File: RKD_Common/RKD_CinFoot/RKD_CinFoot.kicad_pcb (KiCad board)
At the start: 2 copper layers, 81 x 11.9 mm, 5 parts

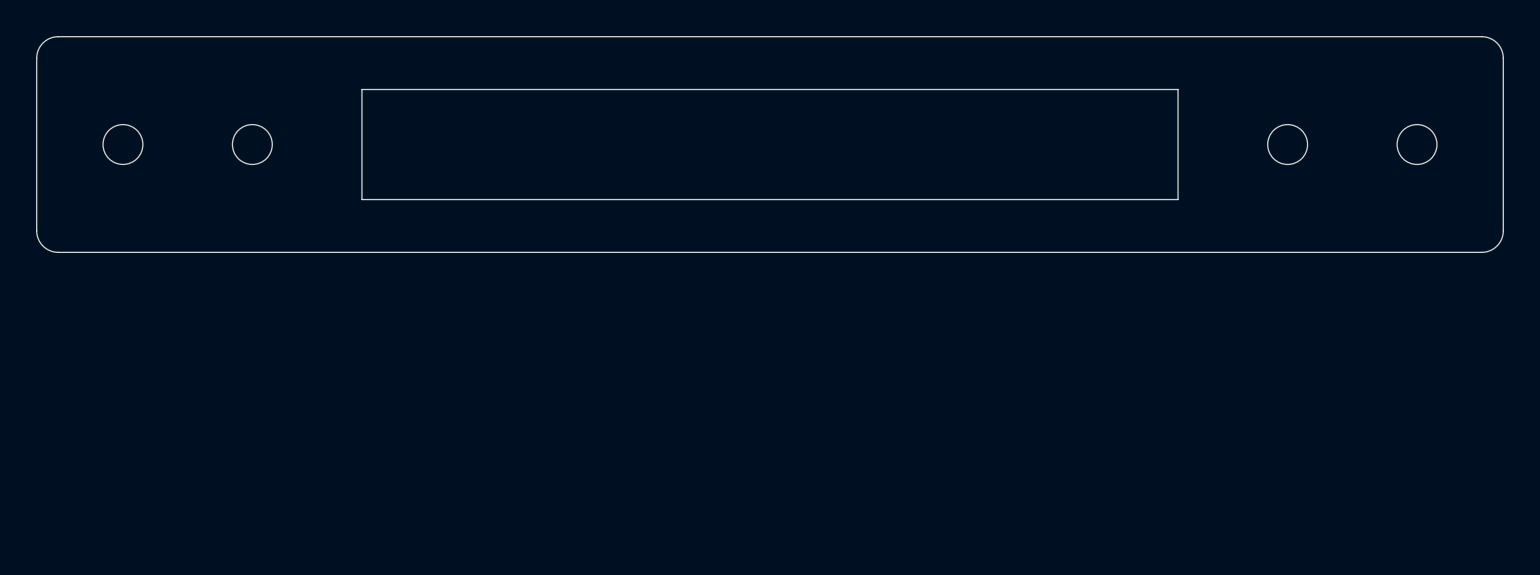
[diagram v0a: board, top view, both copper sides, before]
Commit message: Common UpdateFootPrint
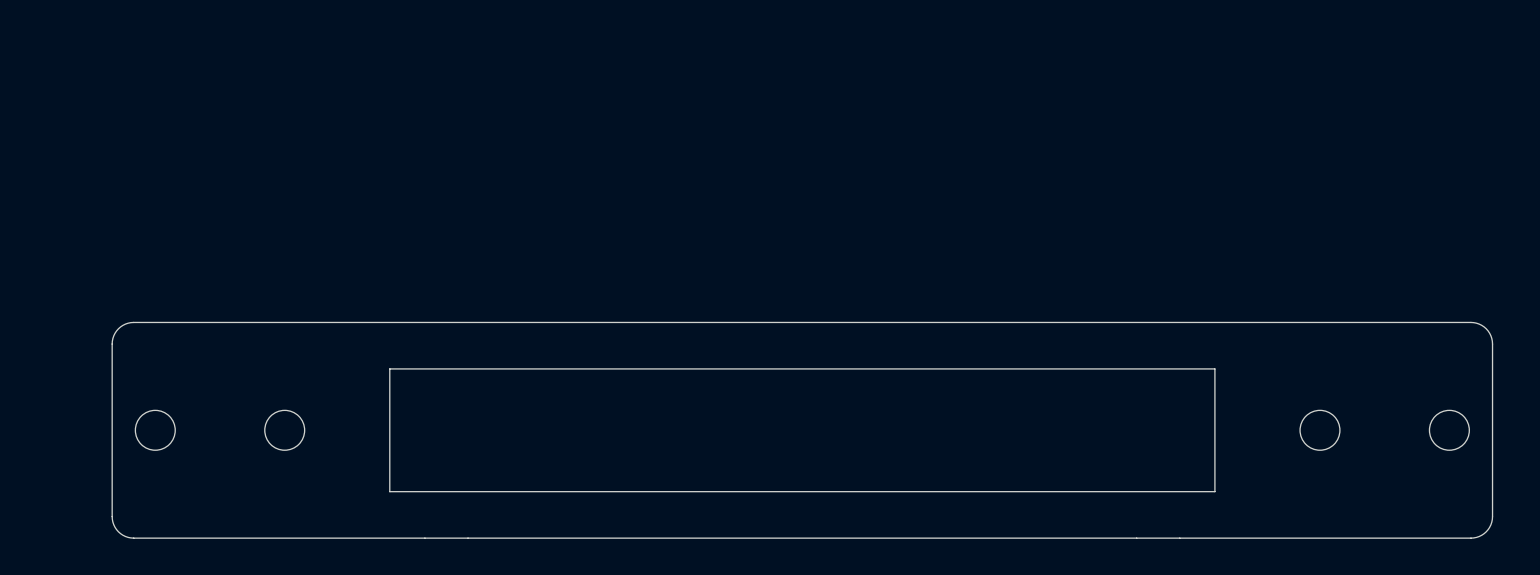
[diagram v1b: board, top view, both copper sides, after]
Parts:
- removed the Ref** at (128.6, 51.2)
- removed the Ref** at (121.4, 51.2)
- removed the Ref** at (64.3, 51.2)
- removed the Ref** at (57.1, 51.2)
- added Ref**: Val**, kbd_Hole:m2_Screw_Hole, F.Cu at (123.2, 67.0)
- added Ref**: Val**, kbd_Hole:m2_Screw_Hole, F.Cu at (58.9, 67.0)
- added Ref**: Val**, kbd_Hole:m2_Screw_Hole, F.Cu at (66.1, 67.0)
- added Ref**: Val**, kbd_Hole:m2_Screw_Hole, F.Cu at (130.4, 67.0)
- moved LED3 15.9 mm to (94.7, 67.0)
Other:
- board size 81 x 11.9 mm -> 76.2 x 11.9 mm
- board text added: "RKD_CinderellaFoot v1.0"
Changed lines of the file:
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@@
 	(footprint "kbd_Hole:m2_Screw_Hole"
 		(layer "F.Cu")
-		(at 128.5875 51.196875)
+		(at 123.229892 66.972702)
 		(descr "Mounting Hole 2.2mm, no annular, M2")
 		(tags "mounting hole 2.2mm no annular m2")
@@
 	(footprint "kbd_Hole:m2_Screw_Hole"
 		(layer "F.Cu")
-		(at 121.44375 51.196875)
+		(at 58.936142 66.972702)
 		(descr "Mounting Hole 2.2mm, no annular, M2")
 		(tags "mounting hole 2.2mm no annular m2")
@@
 	(footprint "kbd_Hole:m2_Screw_Hole"
 		(layer "F.Cu")
-		(at 64.29375 51.196875)
+		(at 66.079892 66.972702)
 		(descr "Mounting Hole 2.2mm, no annular, M2")
 		(tags "mounting hole 2.2mm no annular m2")
@@
 		)
 	)
+	(footprint "Rikkodo_FootPrint:rkd_KeyHall_6wx45_Cinderella"
+		(layer "F.Cu")
+		(at 94.654952 66.972702)
+		(property "Reference" "LED3"
+			(at 6 0.5 0)
+			(layer "F.SilkS")
+			(hide yes)
+			(effects
+				(font
+					(size 1 1)
+					(thickness 0.15)
+				)
+			)
+		)
+		(property "Value" "LED_SK6812MINI-E"
+			(at -5.5 -0.5 0)
+			(layer "F.Fab")
+			(hide yes)
+			(effects
+				(font
+					(size 1 1)
+					(thickness 0.15)
+				)
+			)
+		)
+		(property "Footprint" "Rikkodo_FootPrint:rkd_KeyHall_6wx45_Cinderella"
+			(at 0 0 0)
+			(layer "F.Fab")
+			(hide yes)
+			(effects
+				(font
+					(size 1.27 1.27)
+					(thickness 0.15)
+				)
+			)
+		)
+		(property "Datasheet" ""
+			(at 0 0 0)
+			(layer "F.Fab")
+			(hide yes)
+			(effects
+				(font
+					(size 1.27 1.27)
+					(thickness 0.15)
+				)
+			)
+		)
+		(property "Description" ""
+			(at 0 0 0)
+			(layer "F.Fab")
+			(hide yes)
+			(effects
+				(font
+					(size 1.27 1.27)
+					(thickness 0.15)
+				)
+			)
+		)
+		(attr through_hole)
+		(fp_line
+			(start -22.775 3.3875)
+			(end -22.775 -3.3875)
+			(stroke
+				(width 0.05)
+				(type default)
+			)
+			(layer "Edge.Cuts")
+		)
+		(fp_line
+			(start 22.775 -3.3875)
+			(end -22.775 -3.3875)
+			(stroke
+				(width 0.05)
+				(type default)
+			)
+			(layer "Edge.Cuts")
+		)
+		(fp_line
+			(start 22.775 -3.3875)
+			(end 22.775 3.3875)
+			(stroke
+				(width 0.05)
+				(type default)
+			)
+			(layer "Edge.Cuts")
+		)
+		(fp_line
+			(start 22.775 3.3875)
+			(end -22.775 3.3875)
+			(stroke
+				(width 0.05)
+				(type default)
+			)
+			(layer "Edge.Cuts")
+		)
+	)
 	(footprint "kbd_Hole:m2_Screw_Hole"
 		(layer "F.Cu")
-		(at 57.15 51.196875)
+		(at 130.373642 66.972702)
 		(descr "Mounting Hole 2.2mm, no annular, M2")
 		(tags "mounting hole 2.2mm no annular m2")
@@
 		)
 	)
-	(footprint "Rikkodo_FootPrint:rkd_KeyHall_6wx45_Cinderella"
-		(layer "F.Cu")
-		(at 92.86875 51.196875)
-		(property "Reference" "LED3"
-			(at 6 0.5 0)
-			(layer "F.SilkS")
-			(hide yes)
-			(effects
-				(font
-					(size 1 1)
-					(thickness 0.15)
-				)
-			)
-		)
-		(property "Value" "LED_SK6812MINI-E"
-			(at -5.5 -0.5 0)
-			(layer "F.Fab")
-			(hide yes)
-			(effects
-				(font
-					(size 1 1)
-					(thickness 0.15)
-				)
-			)
-		)
-		(property "Footprint" "Rikkodo_FootPrint:rkd_KeyHall_6wx45_Cinderella"
-			(at 0 0 0)
-			(layer "F.Fab")
-			(hide yes)
-			(effects
-				(font
-					(size 1.27 1.27)
-					(thickness 0.15)
-				)
-			)
-		)
-		(property "Datasheet" ""
-			(at 0 0 0)
-			(layer "F.Fab")
-			(hide yes)
-			(effects
-				(font
-					(size 1.27 1.27)
-					(thickness 0.15)
-				)
-			)
-		)
-		(property "Description" ""
-			(at 0 0 0)
-			(layer "F.Fab")
-			(hide yes)
-			(effects
-				(font
-					(size 1.27 1.27)
-					(thickness 0.15)
-				)
-			)
-		)
-		(attr through_hole)
-		(fp_line
-			(start -22.525 3.0375)
-			(end -22.525 -3.0375)
-			(stroke
-				(width 0.05)
-				(type default)
-			)
-			(layer "Edge.Cuts")
-		)
-		(fp_line
-			(start 22.525 -3.0375)
-			(end -22.525 -3.0375)
-			(stroke
-				(width 0.05)
-				(type default)
-			)
-			(layer "Edge.Cuts")
-		)
-		(fp_line
-			(start 22.525 -3.0375)
-			(end 22.525 3.0375)
-			(stroke
-				(width 0.05)
-				(type default)
-			)
-			(layer "Edge.Cuts")
-		)
-		(fp_line
-			(start 22.525 3.0375)
-			(end -22.525 3.0375)
-			(stroke
-				(width 0.05)
-				(type default)
-			)
-			(layer "Edge.Cuts")
-		)
-	)
 	(gr_arc
-		(start 133.35 55.959375)
-		(mid 133.001274 56.801274)
-		(end 132.159375 57.15)
-		(stroke
-			(width 0.05)
-			(type default)
-		)
-		(layer "Edge.Cuts")
-	)
-	(gr_line
-		(start 132.159375 45.24375)
-		(end 53.578125 45.24375)
+		(start 56.554801 62.210138)
+		(mid 56.903527 61.368239)
+		(end 57.745426 61.019513)
 		(stroke
 			(width 0.05)
@@
 	)
 	(gr_arc
-		(start 52.3875 46.434375)
-		(mid 52.736226 45.592476)
-		(end 53.578125 45.24375)
-		(stroke
-			(width 0.05)
-			(type default)
-		)
-		(layer "Edge.Cuts")
-	)
-	(gr_line
-		(start 132.159375 57.15)
-		(end 53.578125 57.15)
-		(stroke
-			(width 0.05)
-			(type default)
-		)
-		(layer "Edge.Cuts")
-	)
-	(gr_line
-		(start 52.3875 46.434375)
-		(end 52.3875 55.959375)
+		(start 131.564299 61.019573)
+		(mid 132.406196 61.368303)
+		(end 132.754924 62.210198)
 		(stroke
 			(width 0.05)
@@
 	)
 	(gr_arc
-		(start 53.578125 57.15)
-		(mid 52.736226 56.801274)
-		(end 52.3875 55.959375)
+		(start 132.754898 71.7351)
+		(mid 132.406149 72.576979)
+		(end 131.564273 72.925725)
+		(stroke
+			(width 0.05)
+			(type default)
+		)
+		(layer "Edge.Cuts")
+	)
+	(gr_line
+		(start 56.55486 62.210206)
+		(end 56.55486 71.735206)
+		(stroke
+			(width 0.05)
+			(type default)
+		)
+		(layer "Edge.Cuts")
+	)
+	(gr_line
+		(start 131.564299 61.019573)
+		(end 57.745486 61.019572)
+		(stroke
+			(width 0.05)
+			(type default)
+		)
+		(layer "Edge.Cuts")
+	)
+	(gr_line
+		(start 113.109506 72.92572)
+		(end 76.199936 72.92572)
+		(stroke
+			(width 0.05)
+			(type default)
+		)
+		(layer "Edge.Cuts")
+	)
+	(gr_line
+		(start 132.754924 62.210202)
+		(end 132.754924 71.735202)
+		(stroke
+			(width 0.05)
+			(type default)
+		)
+		(layer "Edge.Cuts")
+	)
+	(gr_line
+		(start 73.818684 72.92572)
+		(end 76.199936 72.92572)
+		(stroke
+			(width 0.05)
+			(type default)
+		)
+		(layer "Edge.Cuts")
+	)
+	(gr_line
+		(start 131.564273 72.925725)
+		(end 115.490758 72.92572)
+		(stroke
+			(width 0.05)
+			(type default)
+		)
+		(layer "Edge.Cuts")
+	)
+	(gr_line
+		(start 73.818684 72.92572)
+		(end 57.74551 72.925882)
+		(stroke
+			(width 0.05)
+			(type default)
+		)
+		(layer "Edge.Cuts")
+	)
+	(gr_line
+		(start 113.109506 72.92572)
+		(end 115.490758 72.92572)
 		(stroke
 			(width 0.05)
@@
 	)
 	(gr_arc
-		(start 132.159375 45.24375)
-		(mid 133.001274 45.592476)
-		(end 133.35 46.434375)
-		(stroke
-			(width 0.05)
-			(type default)
-		)
-		(layer "Edge.Cuts")
-	)
-	(gr_line
-		(start 133.35 46.434375)
-		(end 133.35 55.959375)
-		(stroke
-			(width 0.05)
-			(type default)
-		)
-		(layer "Edge.Cuts")
+		(start 57.74551 72.925882)
+		(mid 56.903619 72.577148)
+		(end 56.554885 71.735257)
+		(stroke
+			(width 0.05)
+			(type default)
+		)
+		(layer "Edge.Cuts")
+	)
+	(gr_text "RKD_CinderellaFoot v1.0"
+		(at 126.801768 63.400776 0)
+		(layer "B.SilkS")
+		(effects
+			(font
+				(size 1 1)
+				(thickness 0.1)
+			)
+			(justify left bottom mirror)
+		)
+	)
+	(group ""
+		(members "119e2f71-e038-4129-bcec-3b2945375254" "12d03c72-44ba-4fbf-9bdb-823f6eced25d"
+			"16bad5ad-64f4-4ff5-9c23-298ea4e017e0" "2d08a7a3-aff4-414f-80d4-dfe93a1a73b3"
+			"4b89dfa1-3103-4fc7-b920-419c784dca03" "5400b3c1-3551-4653-a554-9fc24ae7e6c9"
+			"58eba527-2dd0-4d75-a348-94fd6b5970e9" "6916fafc-4c17-4f8d-bbd2-5a074d22d2be"
+			"9630daa5-5a4f-4a8d-a5d8-1ed182757a9f" "a1a3cc95-14b8-4f0b-8d59-1c5646ffd4df"
+			"ad41452a-3768-487e-8399-df2d8a481663" "cc8f9f2b-929e-4d7d-af00-9575b9b466ea"
+			"ce852a84-7158-4034-ae7a-1c5c82d03b17" "d2d7e6a8-f0bb-4800-bf21-3aaf7924e472"
+			"ddc9a58e-fcee-494e-bcdc-0e873c863eda" "e78b853e-3f1f-40d2-b961-3e6054a4ac34"
+			"ecdd45a8-3b2b-41a6-be5a-94f1dfb6cd63" "fe343bde-19ee-4b08-a2df-0cf6b1d1d7c2"
+		)
 	)
 )
